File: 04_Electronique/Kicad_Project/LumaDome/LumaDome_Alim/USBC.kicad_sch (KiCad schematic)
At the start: 25 parts, among them J1 USB_C_Receptacle_PowerOnly_6P, Q1 FDS9435A, U1 CYPD3177-24LQ

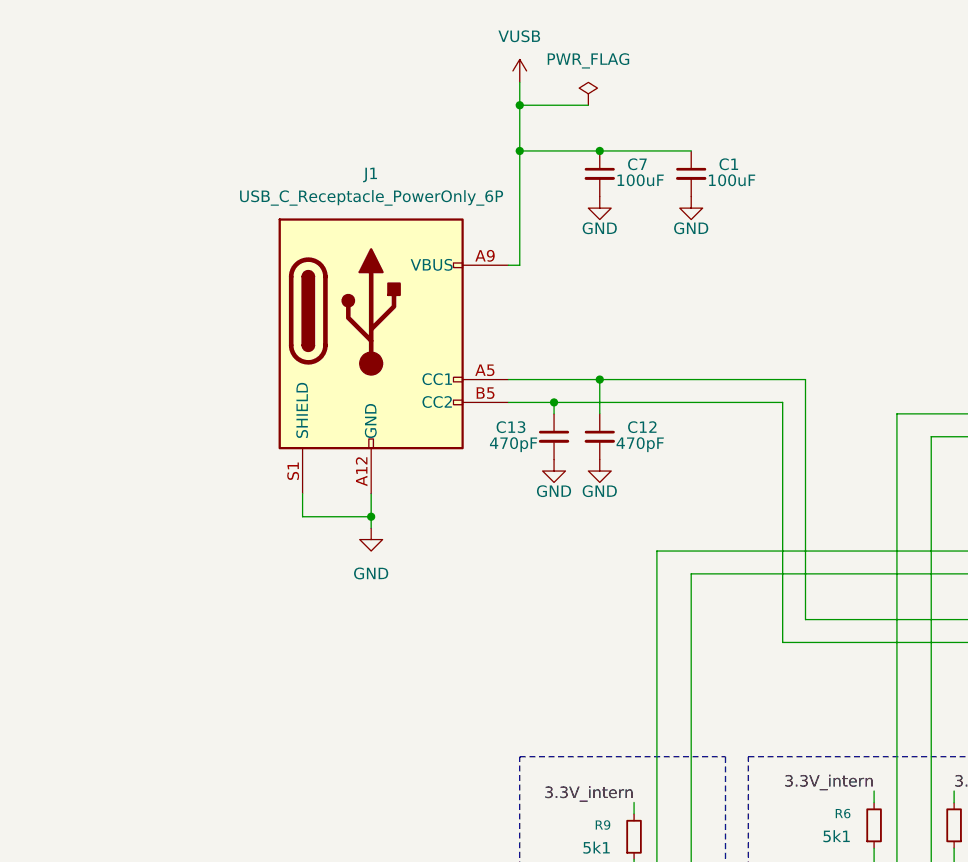
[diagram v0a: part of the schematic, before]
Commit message: finalisation PCB
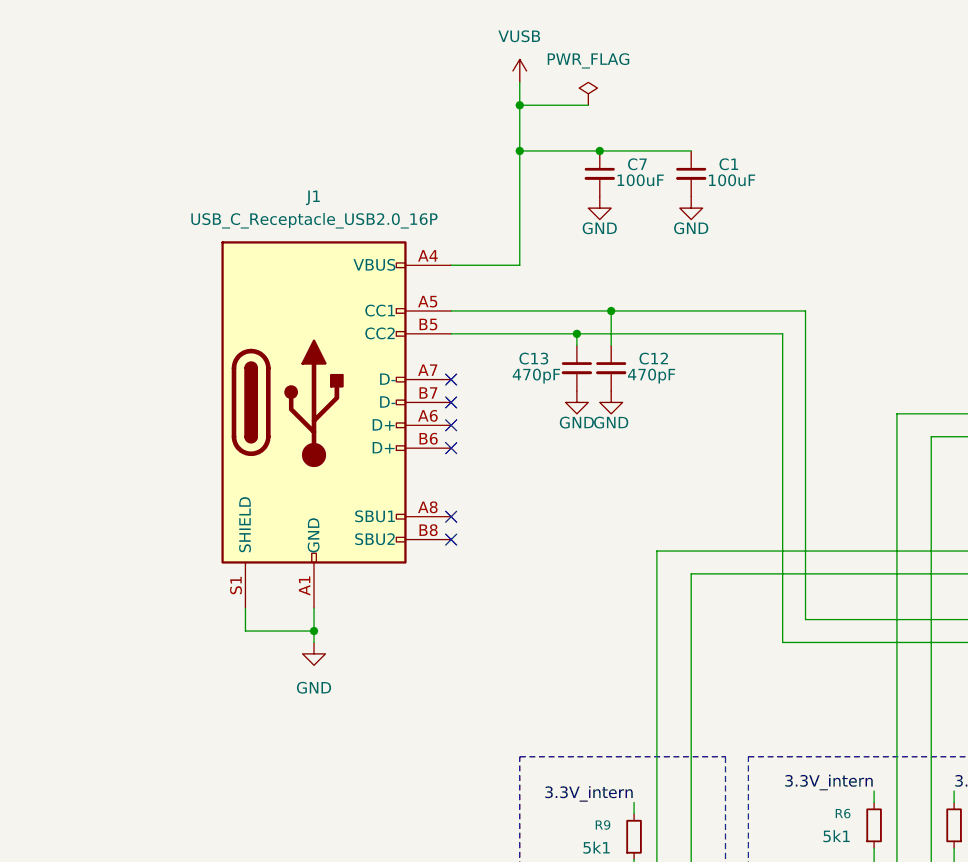
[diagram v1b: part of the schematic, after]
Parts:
- removed J1: USB_C_Receptacle_PowerOnly_6P, Connector_USB:USB_C_Receptacle_GCT_USB4125-xx-x-0190_6P_TopMnt_Horizontal, symbol Connector:USB_C_Receptacle_PowerOnly_6P
- added J1: USB_C_Receptacle_USB2.0_16P, Connector_USB:USB_C_Receptacle_GCT_USB4105-xx-A_16P_TopMnt_Horizontal, symbol Connector:USB_C_Receptacle_USB2.0_16P
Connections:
- net GND: now also J1.A1 (GND), J1.A12 (GND), J1.B1 (GND), J1.B12 (GND), J1.S1 (SHIELD)
- net VUSB: now also J1.A4 (VBUS), J1.A9 (VBUS), J1.B4 (VBUS), J1.B9 (VBUS)
- net at C12.1, U1.15 (CC1): now also J1.A5 (CC1)
- net at C13.1, U1.14 (CC2): now also J1.B5 (CC2)
- no-connect marks 5 -> 11
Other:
- moved on the sheet: C12, C13
